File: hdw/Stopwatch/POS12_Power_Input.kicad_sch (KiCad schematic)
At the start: 19 parts, among them J201 +12V IN, U201 TPS26600RHFT

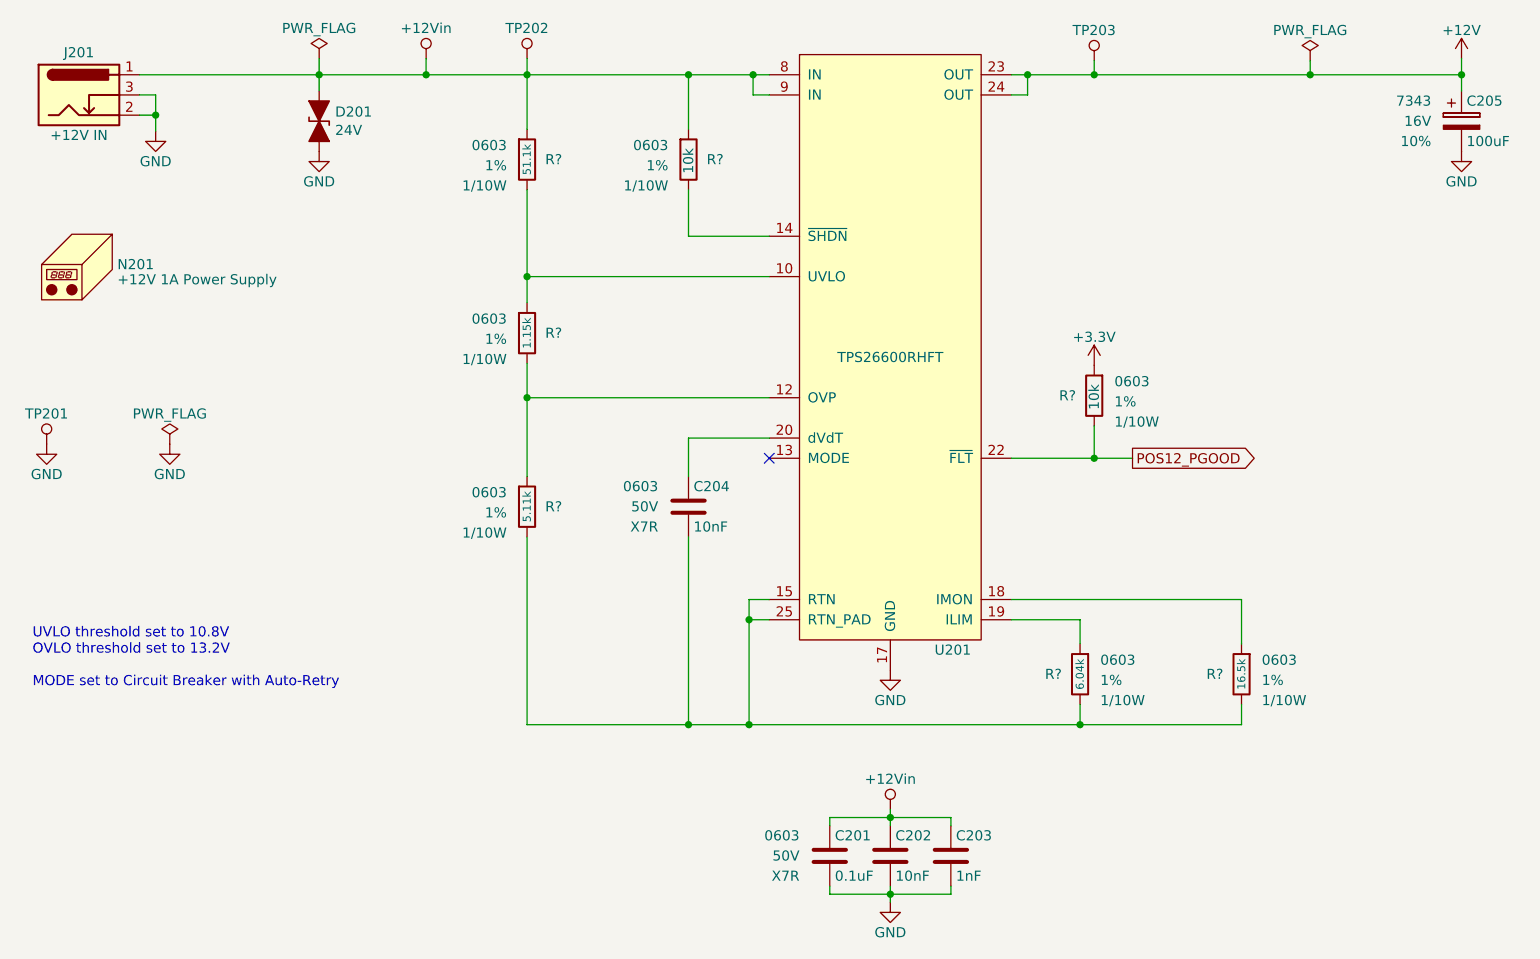
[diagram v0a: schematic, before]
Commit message: started sch work
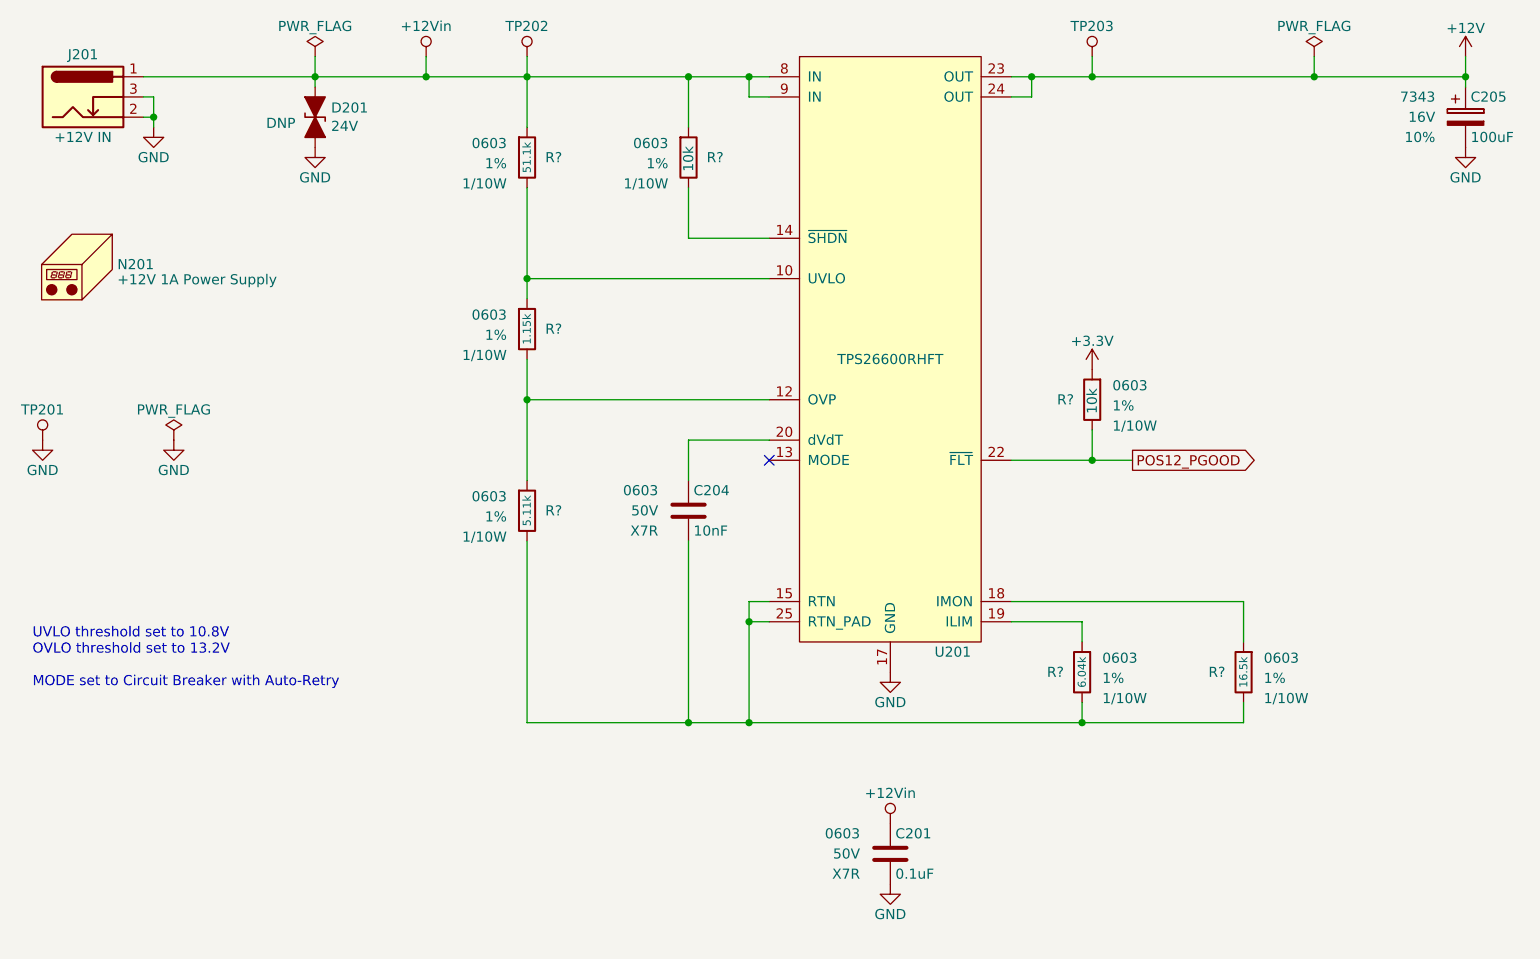
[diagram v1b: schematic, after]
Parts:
- removed C202: 10nF, Capacitors_SMD:C_0603, symbol Custom_Library:C_Custom
- removed C203: 1nF, Capacitors_SMD:C_0603, symbol Custom_Library:C_Custom
- D201: Config (none) -> DNP
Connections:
- net at U201.12 (OVP): now also R?.1, R?.2
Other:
- moved on the sheet: C201, C204, C205, D201, J201, R?, TP201, TP203
